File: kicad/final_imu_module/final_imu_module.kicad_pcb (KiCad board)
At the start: 2 copper layers, 27.5 x 26.5 mm, 15 parts, among them J1 I2C/VDCG, SW1 SW_SPDT, U1 ICM-20948, U2 AMS1117-1.8

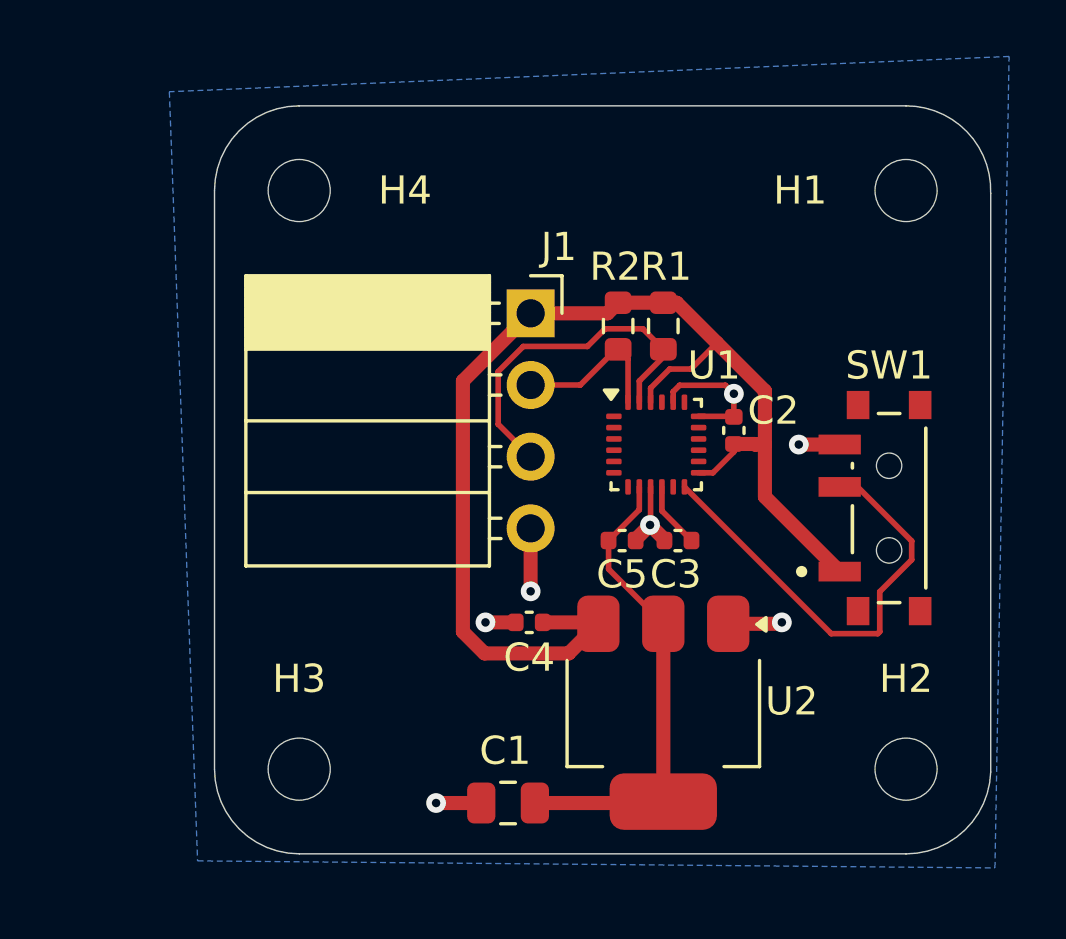
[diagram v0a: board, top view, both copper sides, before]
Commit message: FOINOL DESIGNS
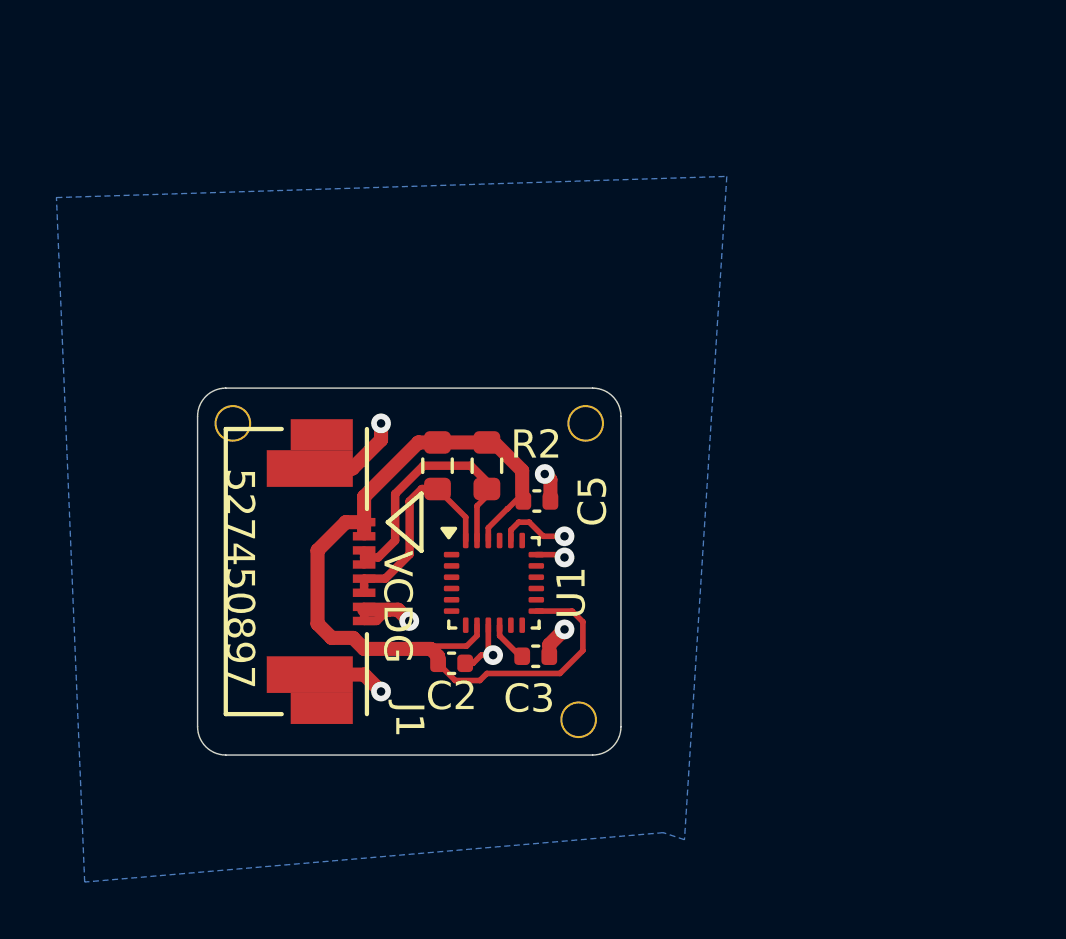
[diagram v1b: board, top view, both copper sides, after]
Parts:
- removed C1: 22u, Capacitor_SMD:C_0805_2012Metric
- removed C4: 10u, Capacitor_SMD:C_0402_1005Metric
- removed H1, H2, H3, H4: MountingHole, MountingHole:MountingHole_2.2mm_M2
- removed SW1: SW_SPDT, external_footprints:SW_SSSS811101
- removed U2: AMS1117-1.8, Package_TO_SOT_SMD:SOT-223-3_TabPin2
- added REF**: tooling_hole, external_footprints:tooling_hole, F.Cu at (102.2, 90.2)
- added REF**: tooling_hole, external_footprints:tooling_hole, F.Cu at (114.8, 90.2)
- added REF**: tooling_hole, external_footprints:tooling_hole, F.Cu at (114.5, 100.8)
- J1: value I2C/VDCG -> 527450897; footprint Connector_PinSocket_2.54mm:PinSocket_1x04_P2.54mm_Horizontal -> external_footprints:CON_527450897_MOL
- moved C2 13.0 mm to (110.0, 98.8), turned to 180 degrees
- moved J1 12.4 mm to (104.5, 95.5), turned to -90 degrees
- moved R1 9.41 mm to (109.5, 91.8)
- moved U1 7.55 mm to (111.5, 95.9)
- moved R2 6.79 mm to (111.2, 91.8)
- moved C3 6.50 mm to (113.0, 98.5), turned to 180 degrees
- moved C5 3.33 mm to (113.0, 93.0)
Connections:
- C2 pad 2: +3.3V -> +1V8
- J1 pad 1: +3.3V -> +1V8
- J1 pad 2: Net-(J1-Pin_2) -> +1V8
- J1 pad 3: Net-(J1-Pin_3) -> Net-(U1-SCL/SCLK)
- J1 pad 4: GND -> Net-(U1-SCL/SCLK)
- R1 pad 1: Net-(J1-Pin_3) -> Net-(U1-SDA/SDI)
- R1 pad 2: +3.3V -> +1V8
- R2 pad 1: Net-(J1-Pin_2) -> Net-(U1-SCL/SCLK)
- R2 pad 2: +3.3V -> +1V8
- U1 pad 12: INT1_OUT -> unconnected-(U1-INT1-Pad12)
- U1 pad 13: +3.3V -> +1V8
- U1 pad 22: +3.3V -> +1V8
- U1 pad 23: Net-(J1-Pin_3) -> Net-(U1-SCL/SCLK)
- U1 pad 24: Net-(J1-Pin_2) -> Net-(U1-SDA/SDI)
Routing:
- net +3.3V: track 43.5 -> 0.00 mm
- net INT1_OUT: track 16.3 -> 0.00 mm
- net +1V8: track 17.0 -> 31.5 mm
- net Net-(J1-Pin_3): track 12.5 -> 0.00 mm
- net Net-(U1-SCL/SCLK): track 0.00 -> 9.83 mm
- net Net-(U1-SDA/SDI): track 0.00 -> 7.83 mm
- net Net-(J1-Pin_2): track 5.64 -> 0.00 mm
- net GND: track 16.0 -> 17.7 mm, vias 7 -> 8
- net Net-(U1-REGOUT): track 2.33 -> 1.47 mm
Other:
- board size 27.5 x 26.5 mm -> 15 x 13 mm
- board text added: "VCDG"
- board text removed: "ICM-20948 PB v1.0"
